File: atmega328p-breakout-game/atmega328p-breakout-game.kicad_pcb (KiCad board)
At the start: 2 copper layers, 77.6 x 52.9 mm, 19 parts, among them J1 Conn_Battery 4.5V, SW1 SW_RESET, SW2 SW_MOVE_RIGHT, SW3 SW_MOVE_LEFT, U1 ATmega328P-P, U2 1088AS

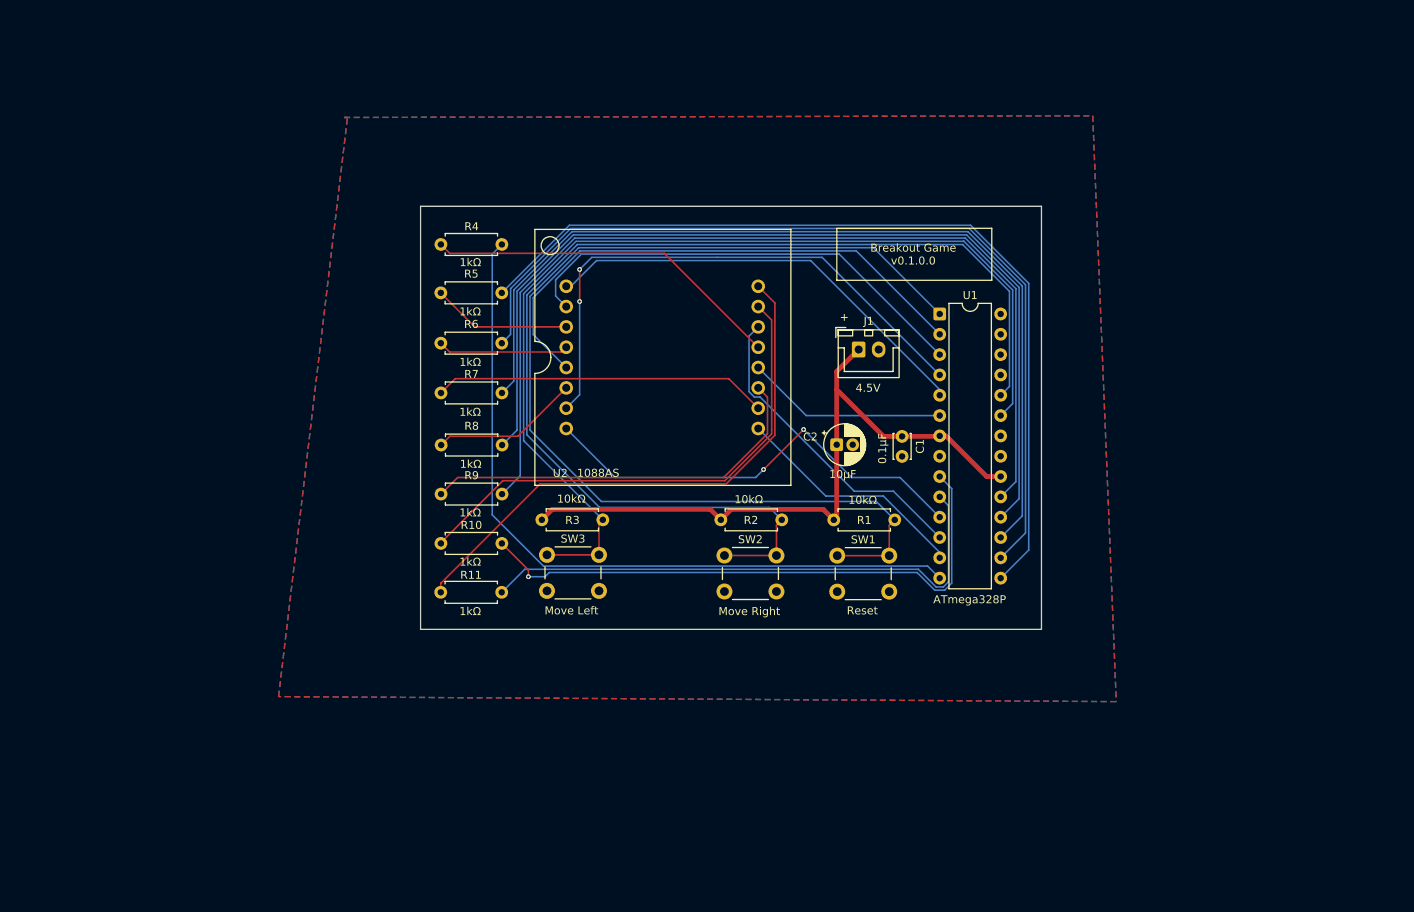
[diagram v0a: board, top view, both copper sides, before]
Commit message: a
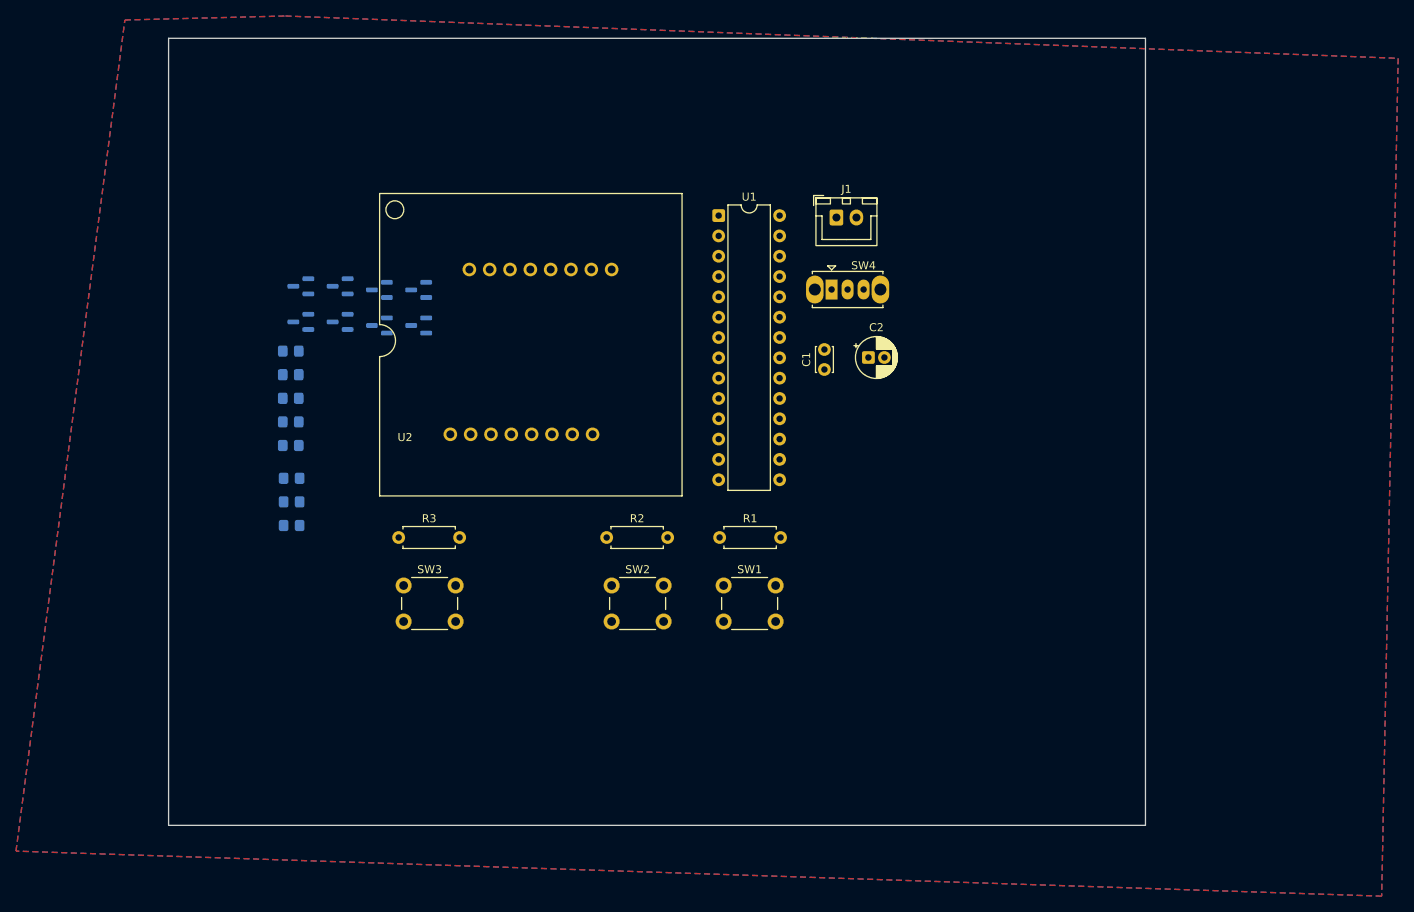
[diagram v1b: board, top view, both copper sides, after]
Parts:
- added Q1: DTC114E, Package_TO_SOT_SMD:SOT-23, B.Cu at (125.9, 79.5)
- added Q2: DTC114E, Package_TO_SOT_SMD:SOT-23, B.Cu at (125.9, 84.0)
- added Q3: DTC114E, Package_TO_SOT_SMD:SOT-23, B.Cu at (121.0, 79.5)
- added Q4: DTC114E, Package_TO_SOT_SMD:SOT-23, B.Cu at (121.0, 84.0)
- added Q5: DTC114E, Package_TO_SOT_SMD:SOT-23, B.Cu at (116.1, 79.1)
- added Q6: DTC114E, Package_TO_SOT_SMD:SOT-23, B.Cu at (116.1, 83.5)
- added Q7: DTC114E, Package_TO_SOT_SMD:SOT-23, B.Cu at (111.2, 79.1)
- added Q8: DTC114E, Package_TO_SOT_SMD:SOT-23, B.Cu at (111.2, 83.5)
- added SW4: SW_DPDT_x2, Button_Switch_THT:SW_Slide_SPDT_Straight_CK_OS102011MS2Q, F.Cu at (177.5, 79.5)
- R10, R11, R4, R5, R6, R7, R8, R9: value 1kΩ -> 220Ω; footprint Resistor_THT:R_Axial_DIN0207_L6.3mm_D2.5mm_P7.62mm_Horizontal -> Resistor_SMD:R_0805_2012Metric_Pad1.20x1.40mm_HandSolder; moved to B.Cu
- U2: value 1088AS -> D15881-M-UR3-0-W; footprint LED_1088:LED_1088 -> LED_1588:LED_1588
- moved R4 39.3 mm to (110.0, 103.1)
- moved R11 32.1 mm to (109.9, 99.0)
- moved R5 32.1 mm to (110.0, 106.0), turned to 180 degrees
- moved R10 30.4 mm to (109.9, 96.0)
- moved U1 30.2 mm to (163.4, 70.3)
- moved R6 29.4 mm to (110.0, 109.0), turned to 180 degrees
- moved R9 29.0 mm to (109.9, 93.1)
- moved R7 26.9 mm to (109.9, 87.2)
- moved R8 20.8 mm to (109.9, 90.2), turned to 180 degrees
- moved U2 19.9 mm to (121.0, 67.5)
- moved SW3 18.3 mm to (124.0, 116.5)
- moved R3 18.0 mm to (123.4, 110.5)
- moved J1 16.7 mm to (178.1, 70.5)
- moved SW1 14.7 mm to (164.0, 116.5)
- moved SW2 14.6 mm to (150.0, 116.5)
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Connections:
- J1 pad 1: VCC -> Net-(J1-Pin_1)
- R10 pad 1: /MATRIX_LED_ROW_7_PIN -> /PORTD5
- R10 pad 2: Net-(U2-R7) -> Net-(U2-C6)
- R11 pad 1: /MATRIX_LED_ROW_8_PIN -> /PORTD6
- R11 pad 2: Net-(U2-R8) -> Net-(U2-C4)
- R4 pad 1: /MATRIX_LED_ROW_1_PIN -> Net-(U2-C2)
- R4 pad 2: Net-(U2-R1) -> /PORTB2
- R5 pad 1: Net-(U2-R2) -> Net-(U2-C3)
- R5 pad 2: /MATRIX_LED_ROW_2_PIN -> /PORTB3
- R6 pad 1: Net-(U2-R3) -> Net-(U2-C5)
- R6 pad 2: /MATRIX_LED_ROW_3_PIN -> /PORTB5
- R7 pad 1: /MATRIX_LED_ROW_4_PIN -> /PORTD0
- R7 pad 2: Net-(U2-R4) -> Net-(U2-C8)
- R8 pad 1: Net-(U2-R5) -> /PORTD1
- R8 pad 2: /MATRIX_LED_ROW_5_PIN -> Net-(U2-C7)
- R9 pad 1: /MATRIX_LED_ROW_6_PIN -> /PORTD3
- R9 pad 2: Net-(U2-R6) -> Net-(U2-C1)
- U1 pad 10: /MATRIX_LED_ROW_8_PIN -> /PORTB7
- U1 pad 11: /MATRIX_LED_COL_6_PIN -> /PORTD5
- U1 pad 12: /MATRIX_LED_COL_7_PIN -> /PORTD6
- U1 pad 13: /MATRIX_LED_COL_8_PIN -> /PORTD7
- U1 pad 14: /MATRIX_LED_ROW_1_PIN -> /PORTB0
- U1 pad 15: /MATRIX_LED_ROW_2_PIN -> /PORTB1
- U1 pad 16: /MATRIX_LED_ROW_3_PIN -> /PORTB2
- U1 pad 17: /MATRIX_LED_ROW_4_PIN -> /PORTB3
- U1 pad 18: /MATRIX_LED_ROW_5_PIN -> /PORTB4
- U1 pad 19: /MATRIX_LED_ROW_6_PIN -> /PORTB5
- U1 pad 2: /MATRIX_LED_COL_1_PIN -> /PORTD0
- U1 pad 3: /MATRIX_LED_COL_2_PIN -> /PORTD1
- U1 pad 4: /MATRIX_LED_COL_3_PIN -> /PORTD2
- U1 pad 5: /MATRIX_LED_COL_4_PIN -> /PORTD3
- U1 pad 6: /MATRIX_LED_COL_5_PIN -> /PORTD4
- U1 pad 9: /MATRIX_LED_ROW_7_PIN -> /PORTB6
- U2 pad 1: /MATRIX_LED_COL_4_PIN -> Net-(Q1-C)
- U2 pad 10: Net-(U2-R4) -> Net-(U2-C4)
- U2 pad 11: Net-(U2-R6) -> Net-(U2-C6)
- U2 pad 12: /MATRIX_LED_COL_5_PIN -> Net-(Q7-C)
- U2 pad 13: Net-(U2-R1) -> Net-(U2-C1)
- U2 pad 14: /MATRIX_LED_COL_7_PIN -> Net-(Q6-C)
- U2 pad 15: Net-(U2-R7) -> Net-(U2-C7)
- U2 pad 16: Net-(U2-R8) -> Net-(U2-C8)
- U2 pad 2: /MATRIX_LED_COL_2_PIN -> Net-(Q2-C)
- U2 pad 3: Net-(U2-R2) -> Net-(U2-C2)
- U2 pad 4: Net-(U2-R3) -> Net-(U2-C3)
- U2 pad 5: /MATRIX_LED_COL_1_PIN -> Net-(Q3-C)
- U2 pad 6: Net-(U2-R5) -> Net-(U2-C5)
- U2 pad 7: /MATRIX_LED_COL_3_PIN -> Net-(Q4-C)
- U2 pad 8: /MATRIX_LED_COL_6_PIN -> Net-(Q5-C)
- U2 pad 9: /MATRIX_LED_COL_8_PIN -> Net-(Q8-C)
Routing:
- net /MOVE_RIGHT_SW: track 143.8 -> 0.00 mm
- net /RESET_SW: track 135.4 -> 0.00 mm
- net /MOVE_LEFT_SW: track 126.1 -> 0.00 mm
- net /MATRIX_LED_ROW_6_PIN: track 120.3 -> 0.00 mm
- net /MATRIX_LED_ROW_5_PIN: track 118.1 -> 0.00 mm
- net /MATRIX_LED_ROW_4_PIN: track 115.4 -> 0.00 mm
- net /MATRIX_LED_ROW_3_PIN: track 113.1 -> 0.00 mm
- net /MATRIX_LED_ROW_2_PIN: track 111.1 -> 0.00 mm
- net /MATRIX_LED_ROW_1_PIN: track 93.5 -> 0.00 mm
- net VCC: track 86.3 -> 0.00 mm
- net /MATRIX_LED_ROW_7_PIN: track 73.9 -> 0.00 mm, vias 1 -> 0
- net Net-(U2-R8): track 70.0 -> 0.00 mm
- net /MATRIX_LED_COL_3_PIN: track 69.8 -> 0.00 mm, vias 2 -> 0
- net /MATRIX_LED_ROW_8_PIN: track 69.3 -> 0.00 mm
- net /MATRIX_LED_COL_1_PIN: track 68.0 -> 0.00 mm
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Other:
- board size 77.6 x 52.9 mm -> 122.1 x 98.4 mm
- board text removed: "+"
- board text removed: "0.1μF"
- board text removed: "1088AS"
- board text removed: "10kΩ"
- board text removed: "10μF"
- board text removed: "1kΩ"
- board text removed: "4.5V"
- board text removed: "ATmega328P"
- board text removed: "Breakout Game v0.1.0.0"
- board text removed: "Move Left"
- board text removed: "Move Right"
- board text removed: "Reset"
